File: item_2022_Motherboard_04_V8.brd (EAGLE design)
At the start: 160 x 100 mm, 130 parts, among them IC1 MCP602SN, IC2 LD117AS33TR, IC3 MCP1525TO, IC4 MCP6S26, IC5 MCP6004SO, IC6 MCP6004SO, IC7 MCP3204SL, IC8 LM336LP, IC9 MCP6004SO, U1 ESP32-DEVKITC-32D, U2 ADS1256_BOARD, U3 SSD1306_128X64, X1 MSTBA4, X2 MSTBA4

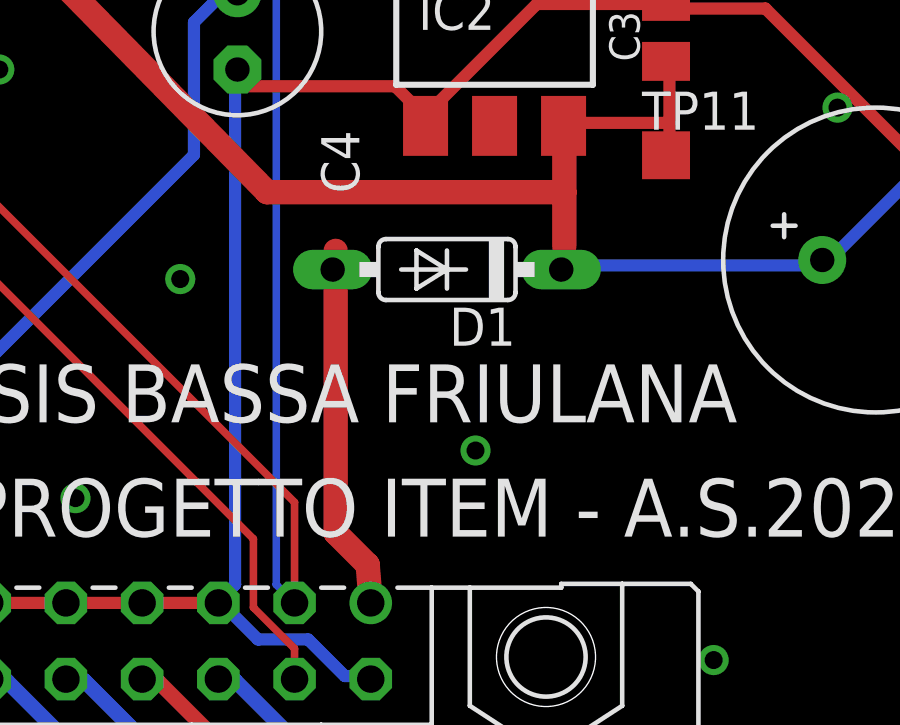
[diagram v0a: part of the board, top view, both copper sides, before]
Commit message: migliorate piste su D1
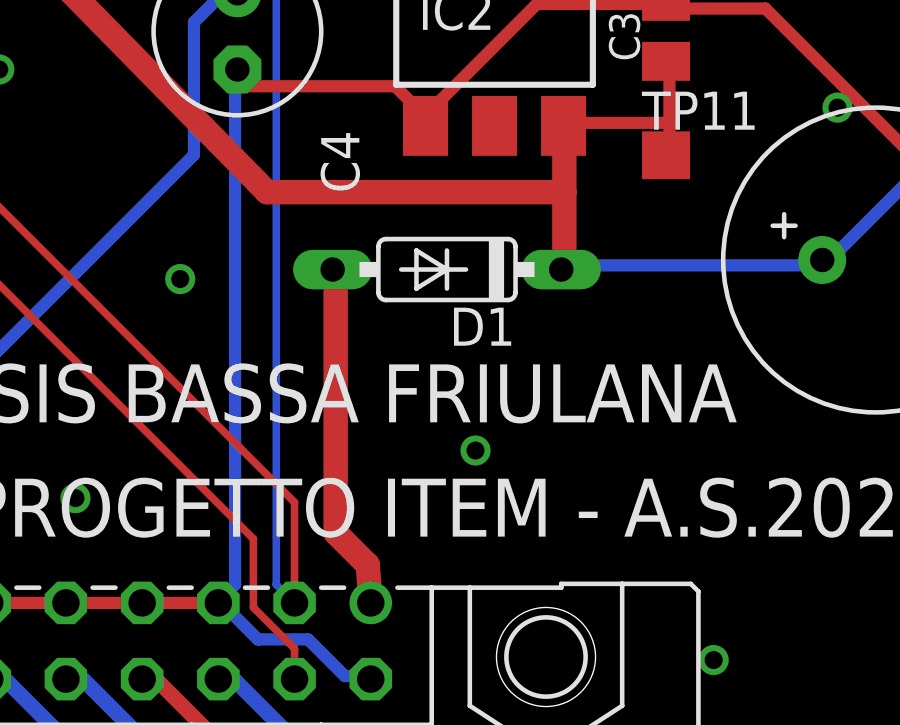
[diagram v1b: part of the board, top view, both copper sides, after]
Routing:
- net EXT_+5V: track 12.8 -> 11.6 mm
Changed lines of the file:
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@@
 <setting verticaltext="up"/>
 </settings>
-<grid distance="0.0125" unitdist="inch" unit="inch" style="lines" multiple="2" display="yes" altdistance="0.025" altunitdist="inch" altunit="inch"/>
+<grid distance="0.0125" unitdist="inch" unit="mm" style="lines" multiple="2" display="yes" altdistance="0.025" altunitdist="inch" altunit="inch"/>
 <layers>
 <layer number="1" name="Top" color="4" fill="1" visible="yes" active="yes"/>
@@
 <layer number="45" name="Holes" color="7" fill="1" visible="no" active="yes"/>
 <layer number="46" name="Milling" color="3" fill="1" visible="no" active="yes"/>
-<layer number="47" name="Measures" color="7" fill="1" visible="no" active="yes"/>
+<layer number="47" name="Measures" color="7" fill="1" visible="yes" active="yes"/>
 <layer number="48" name="Document" color="7" fill="1" visible="no" active="yes"/>
 <layer number="49" name="Reference" color="7" fill="1" visible="no" active="yes"/>
@@
 <wire x1="54.7116" y1="27.432" x2="54.6875" y2="27.33" width="0.4064" layer="1"/>
 <wire x1="54.7116" y1="27.1272" x2="54.7116" y2="25.1206" width="0.8128" layer="1"/>
-<wire x1="54.7116" y1="25.1206" x2="54.7116" y2="23.3172" width="0.8128" layer="1"/>
-<wire x1="54.7116" y1="23.3172" x2="54.61" y2="22.5425" width="0.4064" layer="1"/>
+<wire x1="54.7116" y1="25.1206" x2="54.7116" y2="22.6822" width="0.8128" layer="1"/>
+<wire x1="54.7116" y1="22.6822" x2="54.61" y2="22.5425" width="0.4064" layer="1"/>
 <wire x1="54.7116" y1="27.1272" x2="54.6875" y2="27.33" width="0.4064" layer="1"/>
 <wire x1="29.5275" y1="45.1104" x2="16.6116" y2="45.1104" width="0.8128" layer="1"/>
@@
 <contactref element="D1" pad="A"/>
 <contactref element="PL1" pad="1"/>
-<wire x1="47.0916" y1="13.7668" x2="47.0916" y2="23.1648" width="0.8128" layer="1"/>
+<wire x1="47.0916" y1="13.7668" x2="47.0916" y2="22.5298" width="0.8128" layer="1"/>
 <wire x1="48.1584" y1="12.7" x2="47.0916" y2="13.7668" width="0.8128" layer="1"/>
-<wire x1="47.0916" y1="23.1648" x2="46.99" y2="22.5425" width="0.4064" layer="1"/>
+<wire x1="47.0916" y1="22.5298" x2="46.99" y2="22.5425" width="0.4064" layer="1"/>
 <wire x1="48.1584" y1="12.7" x2="48.26" y2="11.43" width="0.8128" layer="1"/>
 </signal>
